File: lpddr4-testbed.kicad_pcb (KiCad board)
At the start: 6 copper layers, 69.6 x 30 mm, 68 parts, among them IC1 PCA6408APW, IC2 AT24CS01, J1 ddr4-sodimm-edge-connector, U1 MT53E1G32D2NP-046, U2 TPS613221ADBVT

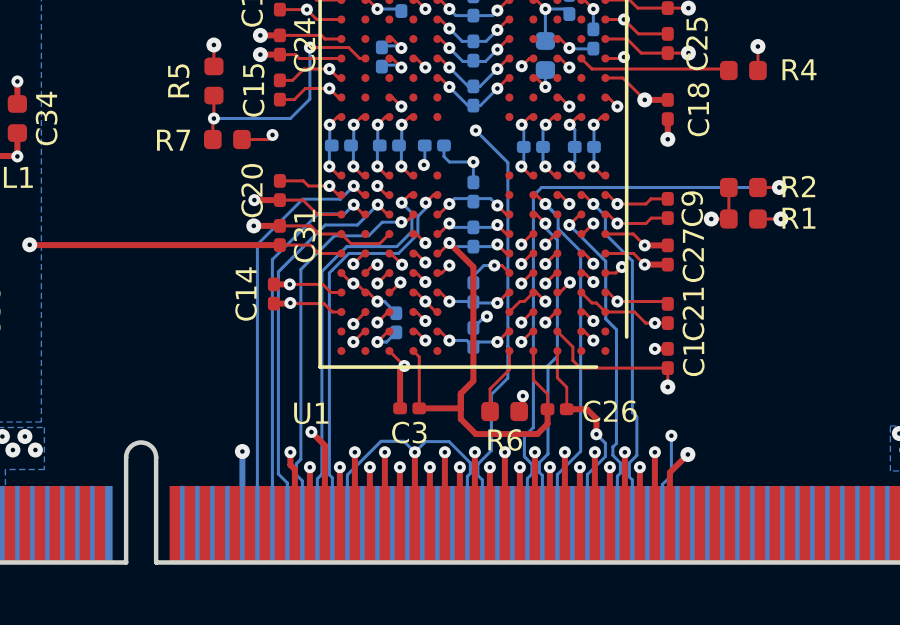
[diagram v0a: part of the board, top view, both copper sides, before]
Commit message: Length matching
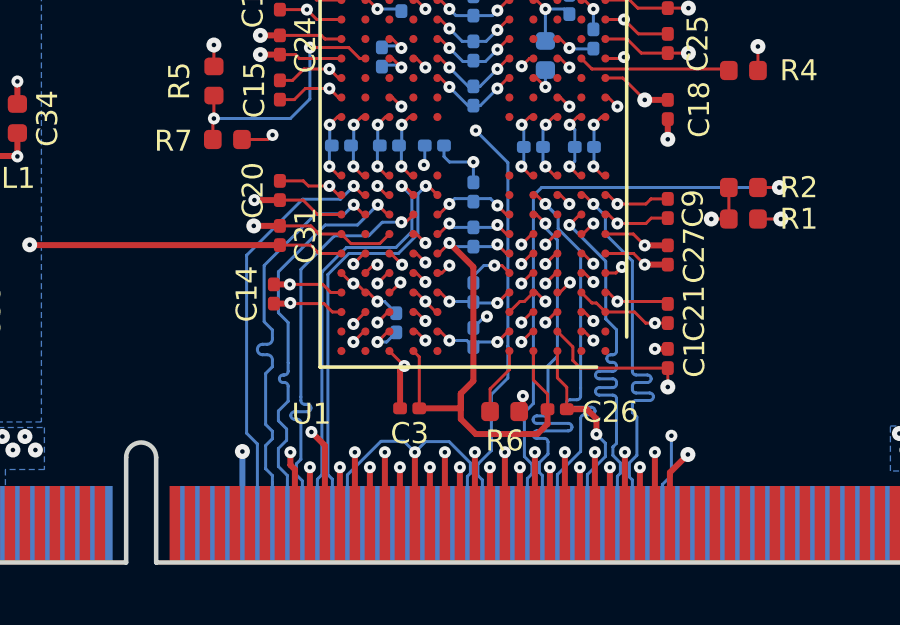
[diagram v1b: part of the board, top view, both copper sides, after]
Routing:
- net CS0_A: track 11.0 -> 14.1 mm
- net DQ_S0_TA: track 13.0 -> 10.2 mm
- net CA0_A: track 11.3 -> 14.1 mm
- net DQ13_A: track 12.7 -> 10.2 mm
- net CA1_A: track 11.9 -> 14.1 mm
- net DQ10_A: track 12.0 -> 10.2 mm
- net CKE0_A: track 12.5 -> 14.1 mm
- net CA4_A: track 12.8 -> 14.1 mm
- net CA2_A: track 13.1 -> 14.1 mm
- net CA3_A: track 13.3 -> 14.1 mm
- net DQ06_A: track 9.44 -> 10.2 mm
- net CK_T_A: track 13.5 -> 14.1 mm
- net DQ09_A: track 10.8 -> 10.2 mm
- net CK_C_A: track 13.6 -> 14.2 mm
- net DQ07_A: track 10.7 -> 10.2 mm
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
